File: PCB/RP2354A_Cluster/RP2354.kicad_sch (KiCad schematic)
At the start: 20 parts, among them U17 RP2340, Y1 12MHz GND24

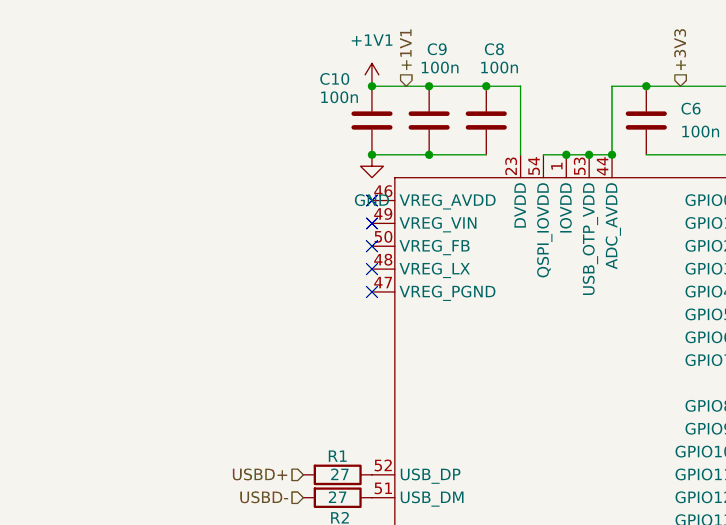
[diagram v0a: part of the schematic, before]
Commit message: fixed power stuff
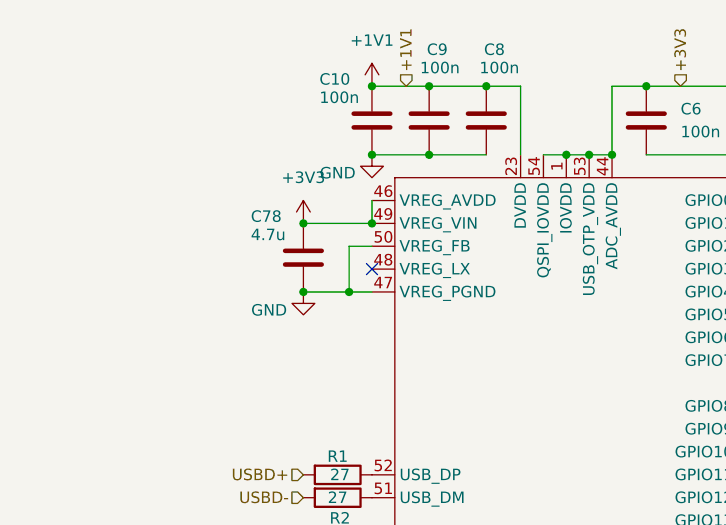
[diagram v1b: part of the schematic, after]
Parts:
- added C78: 4.7u, Basics:C_0402_1005Metric, symbol Device:C
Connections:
- net +3V3: now also U17.46 (VREG_AVDD), U17.49 (VREG_VIN), C78.1
- net GND: now also U17.47 (VREG_PGND), U17.50 (VREG_FB), C78.2
- no-connect marks 10 -> 6
